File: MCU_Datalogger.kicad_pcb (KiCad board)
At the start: 2 copper layers, 29 parts, among them J1 Conn_01x04_Pin, J2 Conn_01x04_Pin, J3 Conn_01x09_Pin, J4 Conn_02x03_Odd_Even, U1 24LC1025, U2 24LC1025, U3 DS1337S_, U4 ATMEGA328P-AU, Y1 32.768 KHz, Y2 16 MHz

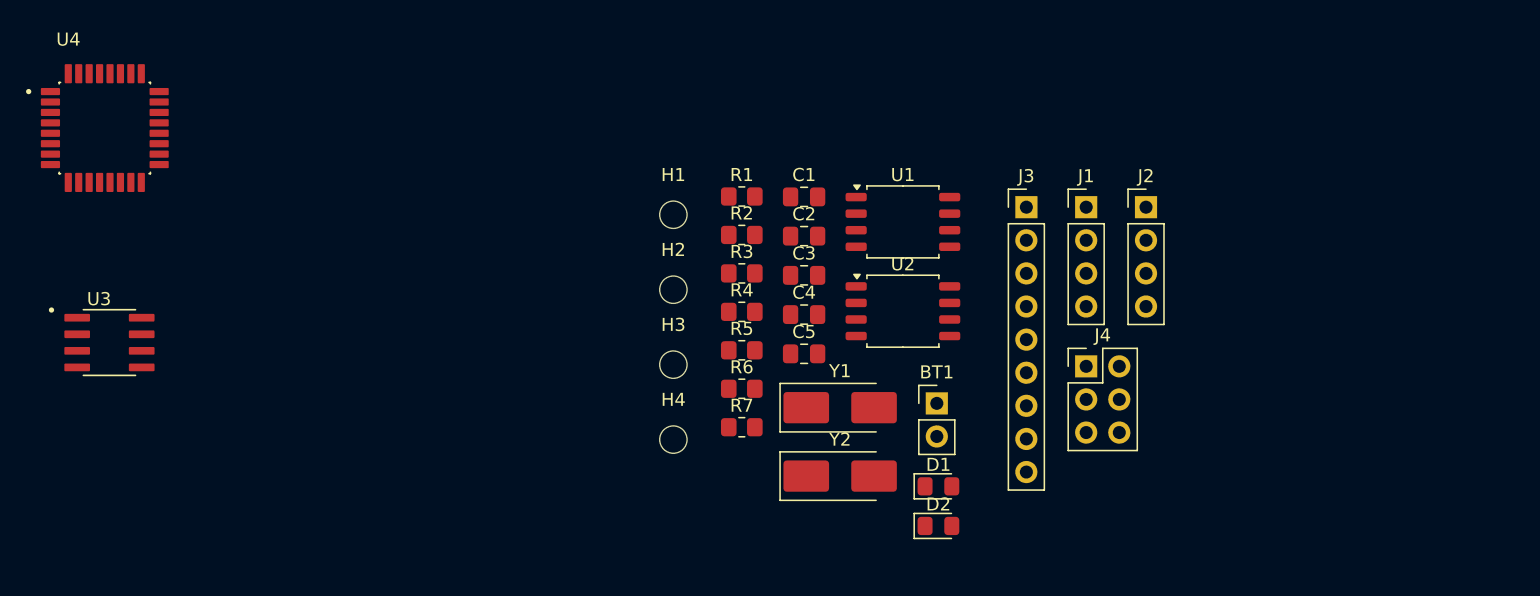
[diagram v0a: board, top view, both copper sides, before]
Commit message: Rout
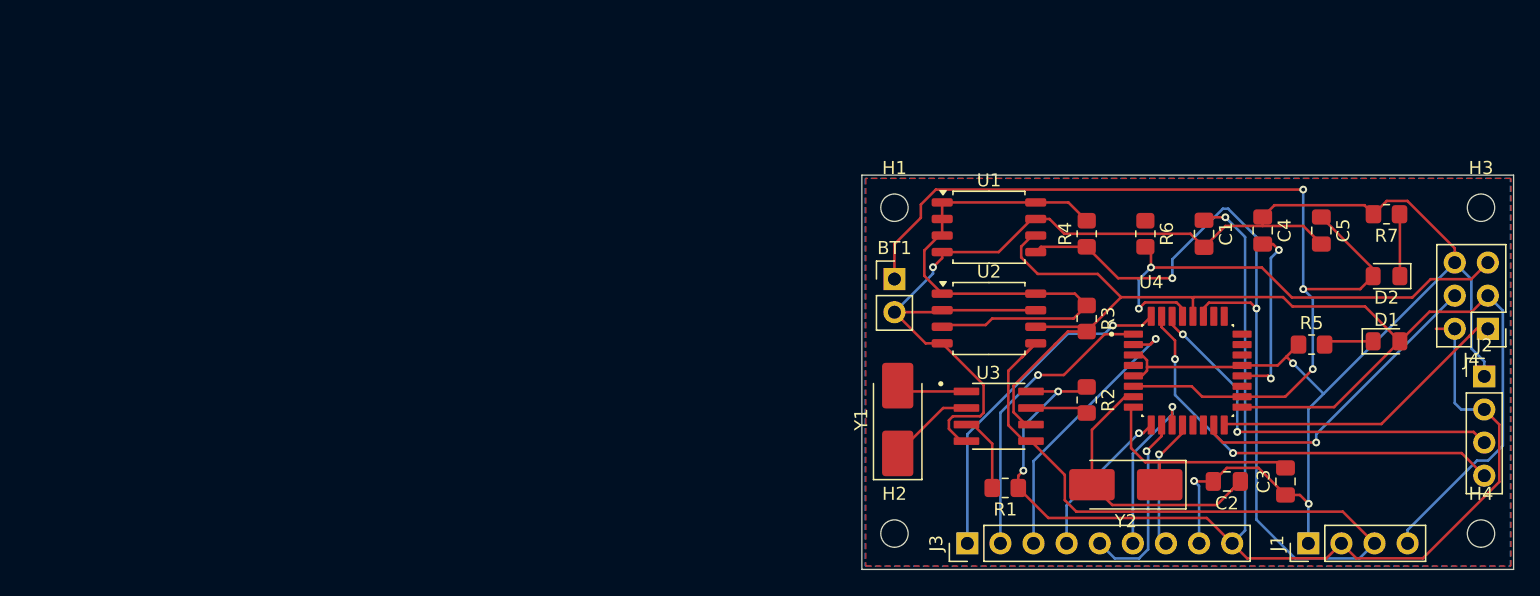
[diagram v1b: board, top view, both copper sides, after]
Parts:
- moved U4 85.1 mm to (162.5, 85.0)
- moved U3 68.5 mm to (148.0, 88.5)
- moved H3 63.1 mm to (185.0, 72.5)
- moved H4 62.4 mm to (185.0, 97.5)
- moved R7 52.1 mm to (177.8, 73.0), turned to 180 degrees
- moved R5 43.7 mm to (172.0, 83.0)
- moved C5 40.8 mm to (172.8, 74.2), turned to -90 degrees
- moved C3 40.2 mm to (170.0, 93.5), turned to 90 degrees
- moved D2 39.4 mm to (177.8, 77.8), turned to 180 degrees
- moved C2 37.5 mm to (165.5, 93.5), turned to 180 degrees
- moved D1 36.1 mm to (177.8, 82.8)
- moved C4 35.8 mm to (168.2, 74.2), turned to -90 degrees
- moved R6 33.2 mm to (159.2, 74.5), turned to -90 degrees
- moved J4 30.9 mm to (185.5, 81.8), turned to 180 degrees
- moved J1 30.9 mm to (171.8, 98.2), turned to 90 degrees
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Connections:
- BT1 pad 1: unconnected-(BT1-+-Pad1) -> Net-(BT1-+)
- BT1 pad 2: unconnected-(BT1---Pad2) -> GND
- C1 pad 1: unconnected-(C1-Pad1) -> /VCC
- C1 pad 2: unconnected-(C1-Pad2) -> GND
- C2 pad 1: unconnected-(C2-Pad1) -> Net-(U4-PB6)
- C2 pad 2: unconnected-(C2-Pad2) -> GND
- C3 pad 1: unconnected-(C3-Pad1) -> GND
- C3 pad 2: unconnected-(C3-Pad2) -> Net-(U4-PB7)
- C4 pad 1: unconnected-(C4-Pad1) -> GND
- C4 pad 2: unconnected-(C4-Pad2) -> Net-(U4-AREF)
- C5 pad 1: unconnected-(C5-Pad1) -> Net-(BT1-+)
- C5 pad 2: unconnected-(C5-Pad2) -> GND
- D1 pad 1: unconnected-(D1-K-Pad1) -> Net-(D1-K)
- D1 pad 2: unconnected-(D1-A-Pad2) -> /SCK
- D2 pad 1: unconnected-(D2-K-Pad1) -> Net-(D2-K)
- D2 pad 2: unconnected-(D2-A-Pad2) -> Net-(BT1-+)
- J1 pad 1: unconnected-(J1-Pin_1-Pad1) -> GND
- J1 pad 2: unconnected-(J1-Pin_2-Pad2) -> /VCC
- J1 pad 3: unconnected-(J1-Pin_3-Pad3) -> /SDA
- J1 pad 4: unconnected-(J1-Pin_4-Pad4) -> /SCK
- J2 pad 1: unconnected-(J2-Pin_1-Pad1) -> GND
- J2 pad 2: unconnected-(J2-Pin_2-Pad2) -> /VCC
- J2 pad 3: unconnected-(J2-Pin_3-Pad3) -> /RX
- J2 pad 4: unconnected-(J2-Pin_4-Pad4) -> /TX
- J3 pad 1: unconnected-(J3-Pin_1-Pad1) -> /D2
- J3 pad 2: unconnected-(J3-Pin_2-Pad2) -> /D3
- J3 pad 3: unconnected-(J3-Pin_3-Pad3) -> /D4
- J3 pad 4: unconnected-(J3-Pin_4-Pad4) -> /D5
- J3 pad 5: unconnected-(J3-Pin_5-Pad5) -> /D6
- J3 pad 6: unconnected-(J3-Pin_6-Pad6) -> /D7
- J3 pad 7: unconnected-(J3-Pin_7-Pad7) -> /D8
- J3 pad 8: unconnected-(J3-Pin_8-Pad8) -> GND
- J3 pad 9: unconnected-(J3-Pin_9-Pad9) -> /VCC
- J4 pad 1: unconnected-(J4-Pin_1-Pad1) -> /MISO
- J4 pad 2: unconnected-(J4-Pin_2-Pad2) -> /VCC
- J4 pad 3: unconnected-(J4-Pin_3-Pad3) -> /SCK
- J4 pad 4: unconnected-(J4-Pin_4-Pad4) -> /MOSI
- J4 pad 5: unconnected-(J4-Pin_5-Pad5) -> /RESET
- J4 pad 6: unconnected-(J4-Pin_6-Pad6) -> GND
- R1 pad 1: unconnected-(R1-Pad1) -> /VCC
- R1 pad 2: unconnected-(R1-Pad2) -> Net-(U3-~{INTA})
- R2 pad 1: unconnected-(R2-Pad1) -> /VCC
- R2 pad 2: unconnected-(R2-Pad2) -> Net-(U3-SQW/~INT)
- R3 pad 1: unconnected-(R3-Pad1) -> /VCC
- R3 pad 2: unconnected-(R3-Pad2) -> /SCK
- R4 pad 1: unconnected-(R4-Pad1) -> /SDA
- R4 pad 2: unconnected-(R4-Pad2) -> /VCC
- R5 pad 1: unconnected-(R5-Pad1) -> GND
- R5 pad 2: unconnected-(R5-Pad2) -> Net-(D1-K)
- R6 pad 1: unconnected-(R6-Pad1) -> /VCC
- R6 pad 2: unconnected-(R6-Pad2) -> /RESET
- R7 pad 1: unconnected-(R7-Pad1) -> Net-(D2-K)
- R7 pad 2: unconnected-(R7-Pad2) -> GND
- U1 pad 1: unconnected-(U1-A0-Pad1) -> /VCC
- U1 pad 2: unconnected-(U1-A1-Pad2) -> /VCC
- U1 pad 3: unconnected-(U1-A2-Pad3) -> /VCC
- U1 pad 4: unconnected-(U1-GND-Pad4) -> GND
- U1 pad 5: unconnected-(U1-SDA-Pad5) -> /SDA
- U1 pad 6: unconnected-(U1-SCL-Pad6) -> /SCK
- U1 pad 7: unconnected-(U1-WP-Pad7) -> GND
- U1 pad 8: unconnected-(U1-VCC-Pad8) -> /VCC
- U2 pad 1: unconnected-(U2-A0-Pad1) -> /VCC
- U2 pad 2: unconnected-(U2-A1-Pad2) -> GND
- U2 pad 3: unconnected-(U2-A2-Pad3) -> /VCC
- U2 pad 4: unconnected-(U2-GND-Pad4) -> GND
- U2 pad 5: unconnected-(U2-SDA-Pad5) -> /SDA
- U2 pad 6: unconnected-(U2-SCL-Pad6) -> /SCK
- U2 pad 7: unconnected-(U2-WP-Pad7) -> GND
- U2 pad 8: unconnected-(U2-VCC-Pad8) -> /VCC
- U3 pad 1: unconnected-(U3-X1-Pad1) -> Net-(U3-X1)
- U3 pad 2: unconnected-(U3-X2-Pad2) -> Net-(U3-X2)
- U3 pad 3: unconnected-(U3-~{INTA}-Pad3) -> Net-(U3-~{INTA})
- U3 pad 4: unconnected-(U3-GND-Pad4) -> GND
- U3 pad 5: unconnected-(U3-SDA-Pad5) -> /SDA
- U3 pad 6: unconnected-(U3-SCL-Pad6) -> /SCK
- U3 pad 7: unconnected-(U3-SQW/~INT-Pad7) -> Net-(U3-SQW/~INT)
- U3 pad 8: unconnected-(U3-VCC-Pad8) -> /VCC
- U4 pad 1: unconnected-(U4-PD3-Pad1) -> /D3
- U4 pad 10: unconnected-(U4-PD6-Pad10) -> /D6
- U4 pad 11: unconnected-(U4-PD7-Pad11) -> /D7
- U4 pad 12: unconnected-(U4-PB0-Pad12) -> /D8
- U4 pad 15: unconnected-(U4-PB3-Pad15) -> /MOSI
- U4 pad 16: unconnected-(U4-PB4-Pad16) -> /MISO
- U4 pad 17: unconnected-(U4-PB5-Pad17) -> /SCK
- U4 pad 18: unconnected-(U4-AVCC-Pad18) -> Net-(BT1-+)
- U4 pad 2: unconnected-(U4-PD4-Pad2) -> /D4
- U4 pad 20: unconnected-(U4-AREF-Pad20) -> Net-(U4-AREF)
- U4 pad 21: unconnected-(U4-GND__2-Pad21) -> GND
- U4 pad 27: unconnected-(U4-PC4-Pad27) -> /SDA
- U4 pad 28: unconnected-(U4-PC5-Pad28) -> /SCK
- U4 pad 29: unconnected-(U4-PC6/~{RESET}-Pad29) -> /RESET
- U4 pad 3: unconnected-(U4-GND-Pad3) -> GND
- U4 pad 30: unconnected-(U4-PD0-Pad30) -> /RX
- U4 pad 31: unconnected-(U4-PD1-Pad31) -> /TX
- U4 pad 32: unconnected-(U4-PD2-Pad32) -> /D2
- U4 pad 5: unconnected-(U4-GND__1-Pad5) -> GND
- U4 pad 6: unconnected-(U4-VCC__1-Pad6) -> Net-(BT1-+)
- U4 pad 7: unconnected-(U4-PB6-Pad7) -> Net-(U4-PB6)
- U4 pad 8: unconnected-(U4-PB7-Pad8) -> Net-(U4-PB7)
- U4 pad 9: unconnected-(U4-PD5-Pad9) -> /D5
- Y1 pad 1: unconnected-(Y1-Pad1) -> Net-(U3-X2)
- Y1 pad 2: unconnected-(Y1-Pad2) -> Net-(U3-X1)
- Y2 pad 1: unconnected-(Y2-Pad1) -> Net-(U4-PB7)
- Y2 pad 2: unconnected-(Y2-Pad2) -> Net-(U4-PB6)
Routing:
- net GND: track 0.00 -> 156.2 mm, vias 0 -> 4
- net /VCC: track 0.00 -> 142.2 mm, vias 0 -> 3
- net /SDA: track 0.00 -> 101.2 mm, vias 0 -> 2
- net /SCK: track 0.00 -> 100.3 mm
- net Net-(BT1-+): track 0.00 -> 77.4 mm, vias 0 -> 3
- net /RESET: track 0.00 -> 37.6 mm, vias 0 -> 2
- net /TX: track 0.00 -> 32.8 mm, vias 0 -> 2
- net /RX: track 0.00 -> 30.3 mm, vias 0 -> 2
- net /D2: track 0.00 -> 26.2 mm, vias 0 -> 1
- net /MOSI: track 0.00 -> 24.5 mm, vias 0 -> 1
- net /MISO: track 0.00 -> 23.7 mm
- net /D3: track 0.00 -> 22.7 mm, vias 0 -> 1
- net /D4: track 0.00 -> 22.7 mm, vias 0 -> 1
- net Net-(U4-PB6): track 0.00 -> 22.2 mm
- net Net-(U4-PB7): track 0.00 -> 17.4 mm
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- added copper zone on F.Cu, net /VCC
- added copper zone on B.Cu, net GND
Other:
- board outline added: 50 x 30.2 mm
